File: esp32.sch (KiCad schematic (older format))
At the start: 18 parts, among them U13 ESP32-WROVER

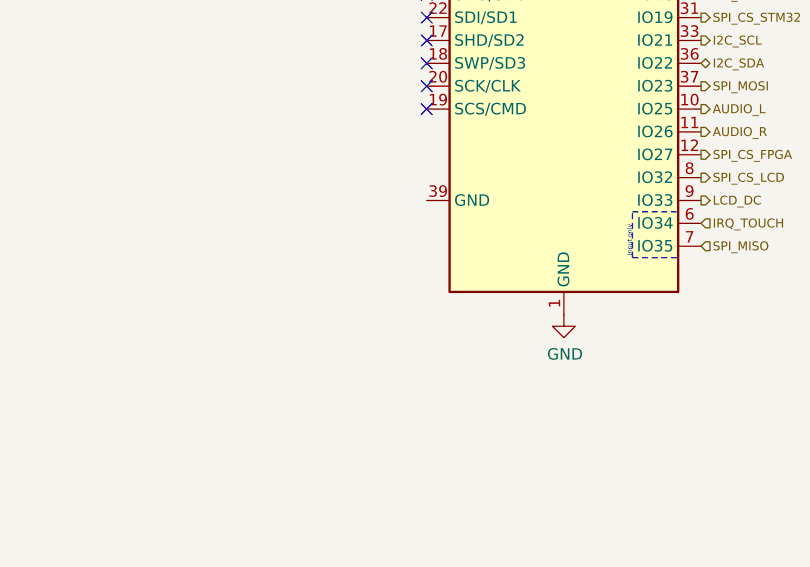
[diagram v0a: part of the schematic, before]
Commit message: Dump.
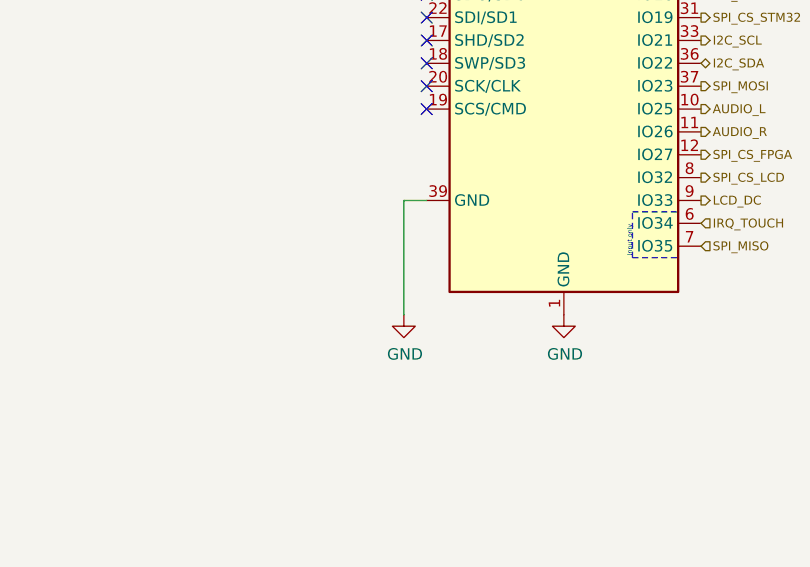
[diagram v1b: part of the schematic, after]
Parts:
- C43: Price 0.0020 -> (none)
- C44: LCSC (none) -> C307461; Price 0.0020 -> (none)
- R46, R49, R60: LCSC - -> C23058; Price 0.0005 -> (none)
- R47, R48, R51, R52, R53, R54, R55, R56, R57, R58: LCSC - -> C115324; Price 0.0005 -> (none)
- R50, R59: Price 0.0005 -> (none)
- U13: Price 0 -> (none)
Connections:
- net GND: now also U13.39 (GND)
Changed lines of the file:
@@
 F 3 "~" H 6150 7300 50  0001 C CNN
 F 4 "C14663" H 6150 7300 50  0001 C CNN "LCSC"
-F 5 "0.0020" H 6150 7300 50  0001 C CNN "Price"
+F 5 "" H 6150 7300 50  0001 C CNN "Price"
 F 6 "-" H 6150 7300 50  0001 C CNN "Mouser"
 F 7 "N" H 6150 7300 50  0001 C CNN "Sponsored"
@@
 F 2 "Capacitor_SMD:C_0603_1608Metric" H 6638 7150 50  0001 C CNN
 F 3 "~" H 6600 7300 50  0001 C CNN
-F 4 "0.0020" H 6600 7300 50  0001 C CNN "Price"
+F 4 "" H 6600 7300 50  0001 C CNN "Price"
 F 5 "N" H 6600 7300 50  0001 C CNN "Sponsored"
+F 6 "C307461" H 6600 7300 50  0001 C CNN "LCSC"
 	1    6600 7300
 	1    0    0    -1
@@
 F 2 "Resistor_SMD:R_0603_1608Metric" V 9730 2250 50  0001 C CNN
 F 3 "~" H 9800 2250 50  0001 C CNN
-F 4 "0.0005" H 9800 2250 50  0001 C CNN "Price"
-F 5 "-" H 9800 2250 50  0001 C CNN "LCSC"
+F 4 "" H 9800 2250 50  0001 C CNN "Price"
+F 5 "C23058" H 9800 2250 50  0001 C CNN "LCSC"
 F 6 "-" H 9800 2250 50  0001 C CNN "Mouser"
 F 7 "N" H 9800 2250 50  0001 C CNN "Sponsored"
@@
 F 2 "Resistor_SMD:R_0603_1608Metric" V 8180 2250 50  0001 C CNN
 F 3 "~" H 8250 2250 50  0001 C CNN
-F 4 "0.0005" H 8250 2250 50  0001 C CNN "Price"
-F 5 "-" H 8250 2250 50  0001 C CNN "LCSC"
+F 4 "" H 8250 2250 50  0001 C CNN "Price"
+F 5 "C23058" H 8250 2250 50  0001 C CNN "LCSC"
 F 6 "-" H 8250 2250 50  0001 C CNN "Mouser"
 F 7 "N" H 8250 2250 50  0001 C CNN "Sponsored"
@@
 F 2 "Resistor_SMD:R_0603_1608Metric" V 9730 1850 50  0001 C CNN
 F 3 "~" H 9800 1850 50  0001 C CNN
-F 4 "0.0005" H 9800 1850 50  0001 C CNN "Price"
+F 4 "" H 9800 1850 50  0001 C CNN "Price"
 F 5 "-" H 9800 1850 50  0001 C CNN "LCSC"
 F 6 "-" H 9800 1850 50  0001 C CNN "Mouser"
@@
 F 2 "Resistor_SMD:R_0603_1608Metric" V 8930 2250 50  0001 C CNN
 F 3 "~" H 9000 2250 50  0001 C CNN
-F 4 "0.0005" H 9000 2250 50  0001 C CNN "Price"
+F 4 "" H 9000 2250 50  0001 C CNN "Price"
 F 5 "-" H 9000 2250 50  0001 C CNN "LCSC"
 F 6 "-" H 9000 2250 50  0001 C CNN "Mouser"
@@
 F 2 "Resistor_SMD:R_0603_1608Metric" V 8930 1850 50  0001 C CNN
 F 3 "~" H 9000 1850 50  0001 C CNN
-F 4 "0.0005" H 9000 1850 50  0001 C CNN "Price"
-F 5 "-" H 9000 1850 50  0001 C CNN "LCSC"
+F 4 "" H 9000 1850 50  0001 C CNN "Price"
+F 5 "C23058" H 9000 1850 50  0001 C CNN "LCSC"
 F 6 "-" H 9000 1850 50  0001 C CNN "Mouser"
 F 7 "N" H 9000 1850 50  0001 C CNN "Sponsored"
@@
 F 2 "custom:ESP32-WROVER" H 3650 2700 50  0001 C CNN
 F 3 "https://www.espressif.com/sites/default/files/documentation/esp32-wroom-32_datasheet_en.pdf" H 3350 4250 50  0001 C CNN
-F 4 "0" H 3650 4200 50  0001 C CNN "Price"
+F 4 "" H 3650 4200 50  0001 C CNN "Price"
 F 5 "-" H 3650 4200 50  0001 C CNN "LCSC"
 F 6 "-" H 3650 4200 50  0001 C CNN "Mouser"
@@
 F 2 "Resistor_SMD:R_0603_1608Metric" V 9680 4750 50  0001 C CNN
 F 3 "~" H 9750 4750 50  0001 C CNN
-F 4 "0.0005" H 9750 4750 50  0001 C CNN "Price"
-F 5 "-" H 9750 4750 50  0001 C CNN "LCSC"
+F 4 "" H 9750 4750 50  0001 C CNN "Price"
+F 5 "C115324" H 9750 4750 50  0001 C CNN "LCSC"
 F 6 "-" H 9750 4750 50  0001 C CNN "Mouser"
 F 7 "N" H 9750 4750 50  0001 C CNN "Sponsored"
@@
 F 2 "Resistor_SMD:R_0603_1608Metric" V 9580 4750 50  0001 C CNN
 F 3 "~" H 9650 4750 50  0001 C CNN
-F 4 "0.0005" H 9650 4750 50  0001 C CNN "Price"
-F 5 "-" H 9650 4750 50  0001 C CNN "LCSC"
+F 4 "" H 9650 4750 50  0001 C CNN "Price"
+F 5 "C115324" H 9650 4750 50  0001 C CNN "LCSC"
 F 6 "-" H 9650 4750 50  0001 C CNN "Mouser"
 F 7 "N" H 9650 4750 50  0001 C CNN "Sponsored"
@@
 F 2 "Resistor_SMD:R_0603_1608Metric" V 9480 4750 50  0001 C CNN
 F 3 "~" H 9550 4750 50  0001 C CNN
-F 4 "0.0005" H 9550 4750 50  0001 C CNN "Price"
-F 5 "-" H 9550 4750 50  0001 C CNN "LCSC"
+F 4 "" H 9550 4750 50  0001 C CNN "Price"
+F 5 "C115324" H 9550 4750 50  0001 C CNN "LCSC"
 F 6 "-" H 9550 4750 50  0001 C CNN "Mouser"
 F 7 "N" H 9550 4750 50  0001 C CNN "Sponsored"
@@
 F 2 "Resistor_SMD:R_0603_1608Metric" V 9380 4750 50  0001 C CNN
 F 3 "~" H 9450 4750 50  0001 C CNN
-F 4 "0.0005" H 9450 4750 50  0001 C CNN "Price"
-F 5 "-" H 9450 4750 50  0001 C CNN "LCSC"
+F 4 "" H 9450 4750 50  0001 C CNN "Price"
+F 5 "C115324" H 9450 4750 50  0001 C CNN "LCSC"
 F 6 "-" H 9450 4750 50  0001 C CNN "Mouser"
 F 7 "N" H 9450 4750 50  0001 C CNN "Sponsored"
@@
 F 2 "Resistor_SMD:R_0603_1608Metric" V 9280 4750 50  0001 C CNN
 F 3 "~" H 9350 4750 50  0001 C CNN
-F 4 "0.0005" H 9350 4750 50  0001 C CNN "Price"
-F 5 "-" H 9350 4750 50  0001 C CNN "LCSC"
+F 4 "" H 9350 4750 50  0001 C CNN "Price"
+F 5 "C115324" H 9350 4750 50  0001 C CNN "LCSC"
 F 6 "-" H 9350 4750 50  0001 C CNN "Mouser"
 F 7 "N" H 9350 4750 50  0001 C CNN "Sponsored"
@@
 F 2 "Resistor_SMD:R_0603_1608Metric" V 9180 4750 50  0001 C CNN
 F 3 "~" H 9250 4750 50  0001 C CNN
-F 4 "0.0005" H 9250 4750 50  0001 C CNN "Price"
-F 5 "-" H 9250 4750 50  0001 C CNN "LCSC"
+F 4 "" H 9250 4750 50  0001 C CNN "Price"
+F 5 "C115324" H 9250 4750 50  0001 C CNN "LCSC"
 F 6 "-" H 9250 4750 50  0001 C CNN "Mouser"
 F 7 "N" H 9250 4750 50  0001 C CNN "Sponsored"
@@
 F 2 "Resistor_SMD:R_0603_1608Metric" V 9080 4750 50  0001 C CNN
 F 3 "~" H 9150 4750 50  0001 C CNN
-F 4 "0.0005" H 9150 4750 50  0001 C CNN "Price"
-F 5 "-" H 9150 4750 50  0001 C CNN "LCSC"
+F 4 "" H 9150 4750 50  0001 C CNN "Price"
+F 5 "C115324" H 9150 4750 50  0001 C CNN "LCSC"
 F 6 "-" H 9150 4750 50  0001 C CNN "Mouser"
 F 7 "N" H 9150 4750 50  0001 C CNN "Sponsored"
@@
 F 2 "Resistor_SMD:R_0603_1608Metric" V 8980 4750 50  0001 C CNN
 F 3 "~" H 9050 4750 50  0001 C CNN
-F 4 "0.0005" H 9050 4750 50  0001 C CNN "Price"
-F 5 "-" H 9050 4750 50  0001 C CNN "LCSC"
+F 4 "" H 9050 4750 50  0001 C CNN "Price"
+F 5 "C115324" H 9050 4750 50  0001 C CNN "LCSC"
 F 6 "-" H 9050 4750 50  0001 C CNN "Mouser"
 F 7 "N" H 9050 4750 50  0001 C CNN "Sponsored"
@@
 F 2 "Resistor_SMD:R_0603_1608Metric" V 8880 4750 50  0001 C CNN
 F 3 "~" H 8950 4750 50  0001 C CNN
-F 4 "0.0005" H 8950 4750 50  0001 C CNN "Price"
-F 5 "-" H 8950 4750 50  0001 C CNN "LCSC"
+F 4 "" H 8950 4750 50  0001 C CNN "Price"
+F 5 "C115324" H 8950 4750 50  0001 C CNN "LCSC"
 F 6 "-" H 8950 4750 50  0001 C CNN "Mouser"
 F 7 "N" H 8950 4750 50  0001 C CNN "Sponsored"
@@
 F 2 "Resistor_SMD:R_0603_1608Metric" V 8780 4750 50  0001 C CNN
 F 3 "~" H 8850 4750 50  0001 C CNN
-F 4 "0.0005" H 8850 4750 50  0001 C CNN "Price"
-F 5 "-" H 8850 4750 50  0001 C CNN "LCSC"
+F 4 "" H 8850 4750 50  0001 C CNN "Price"
+F 5 "C115324" H 8850 4750 50  0001 C CNN "LCSC"
 F 6 "-" H 8850 4750 50  0001 C CNN "Mouser"
 F 7 "N" H 8850 4750 50  0001 C CNN "Sponsored"
@@
 Text HLabel 4250 4300 2    39   Output ~ 0
 SPI_CS_STM32
+Wire Wire Line
+	3050 5100 2950 5100
+$Comp
+L power:GND #PWR0181
+U 1 1 5F69C61B
+P 2950 5600
+F 0 "#PWR0181" H 2950 5350 50  0001 C CNN
+F 1 "GND" H 2955 5427 50  0000 C CNN
+F 2 "" H 2950 5600 50  0001 C CNN
+F 3 "" H 2950 5600 50  0001 C CNN
+	1    2950 5600
+	1    0    0    -1
+$EndComp
+Wire Wire Line
+	2950 5100 2950 5600
 $EndSCHEMATC

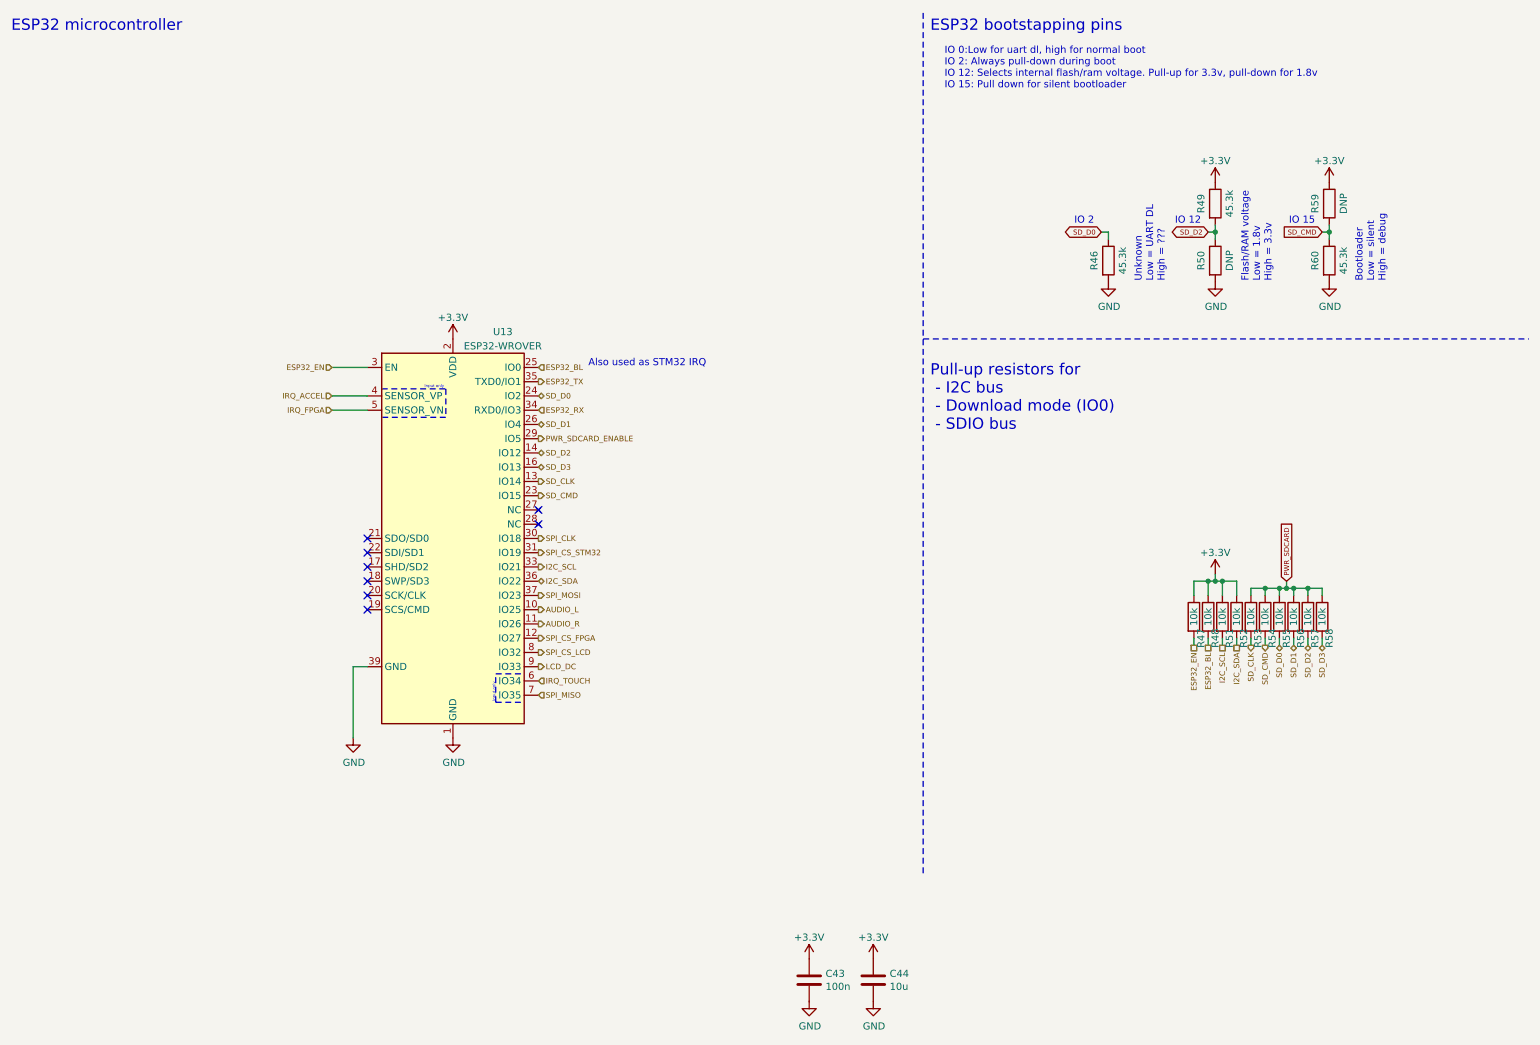
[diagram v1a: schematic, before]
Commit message: Work in progress: prototype 2
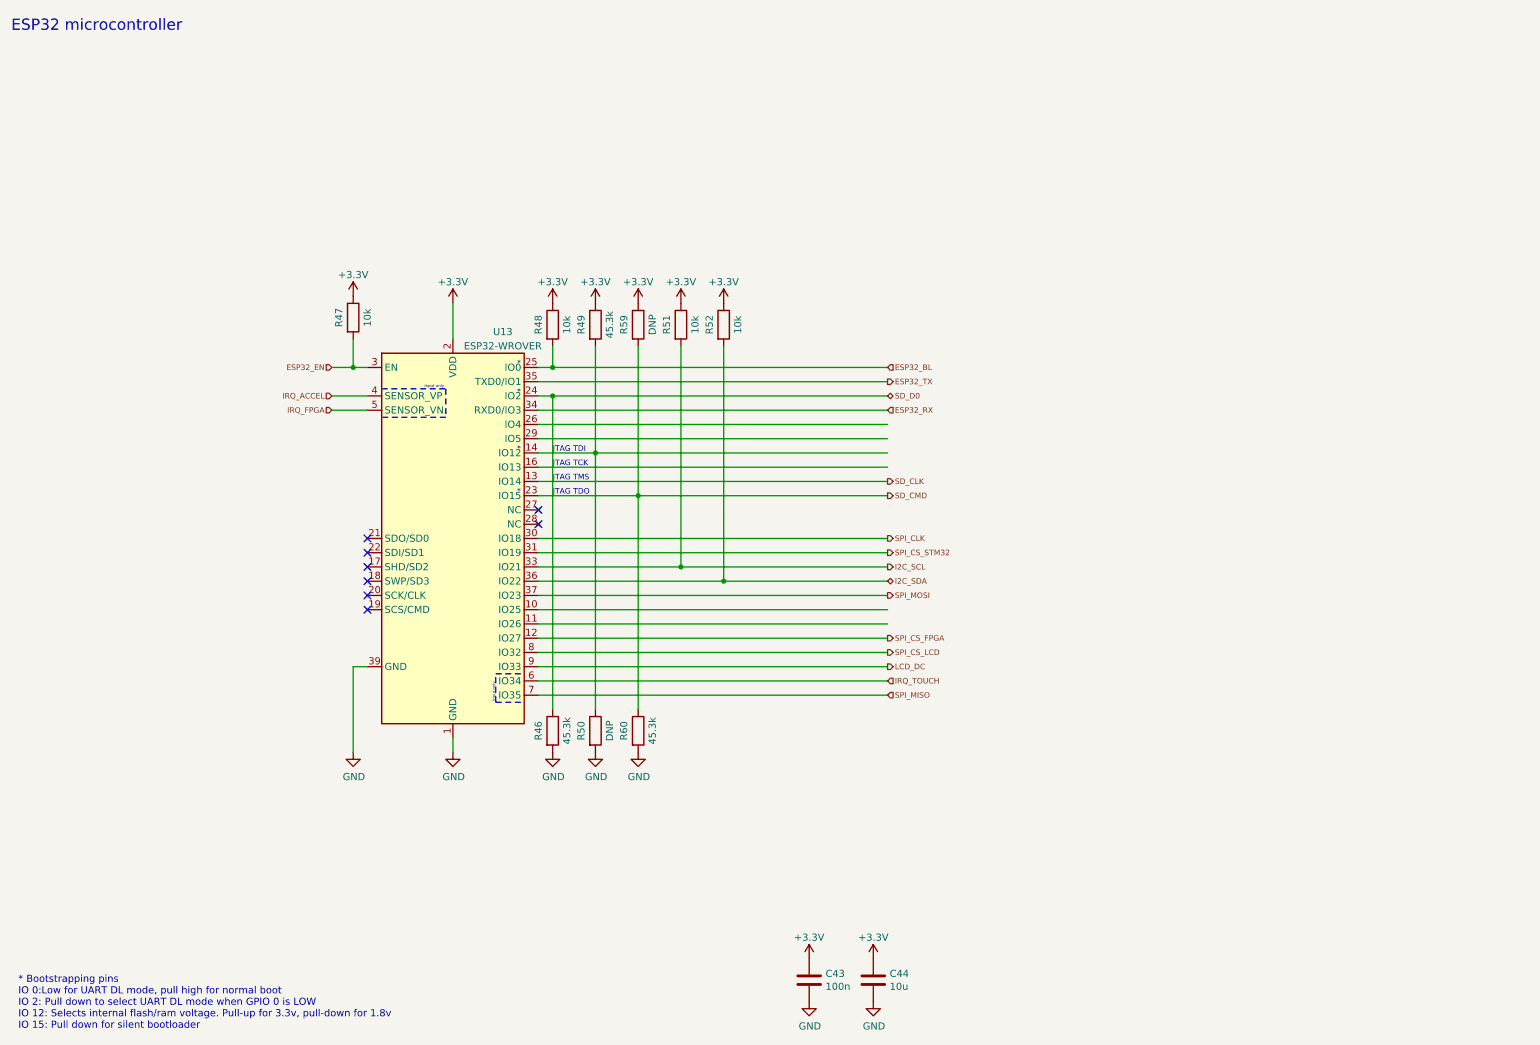
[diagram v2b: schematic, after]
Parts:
- removed R53, R54, R55, R56, R57, R58: 10k, Resistor_SMD:R_0603_1608Metric, symbol Device:R
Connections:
- net labels removed: AUDIO_L, AUDIO_R, PWR_SDCARD, PWR_SDCARD_ENABLE, SD_D1, SD_D2, SD_D3
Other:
- note added: "*"
- note added: "* Bootstrapping pins\nIO 0:Low for UART DL mode, pull high for normal boot\nIO 2: Pull down to select UART DL mode when GPIO 0 is LOW\nIO 12: Selects internal flash/ram voltage. Pull-up for 3.3v, pull-down for 1.8v\nIO 15: Pull down for silent bootloader"
- note added: "JTAG TCK"
- note added: "JTAG TDI"
- note added: "JTAG TDO"
- note added: "JTAG TMS"
- note removed: "Also used as STM32 IRQ"
- note removed: "Bootloader\nLow = silent\nHigh = debug"
- note removed: "ESP32 bootstapping pins"
- note removed: "Flash/RAM voltage\nLow = 1.8v\nHigh = 3.3v"
- note removed: "IO 0:Low for uart dl, high for normal boot\nIO 2: Always pull-down during boot\nIO 12: Selects internal flash/ram voltage. Pull-up for 3.3v, pull-down for 1.8v\nIO 15: Pull down for silent bootloader"
- note removed: "IO 12"
- note removed: "IO 15"
- note removed: "IO 2"
- note removed: "Pull-up resistors for\n - I2C bus\n - Download mode (IO0)\n - SDIO bus"
- note removed: "Unknown\nLow = UART DL\nHigh = ???"
- moved on the sheet: R46, R47, R48, R49, R50, R51, R52, R59, R60
